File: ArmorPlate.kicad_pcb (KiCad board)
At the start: 2 copper layers, 46 parts, among them SW3 SW_SP3T

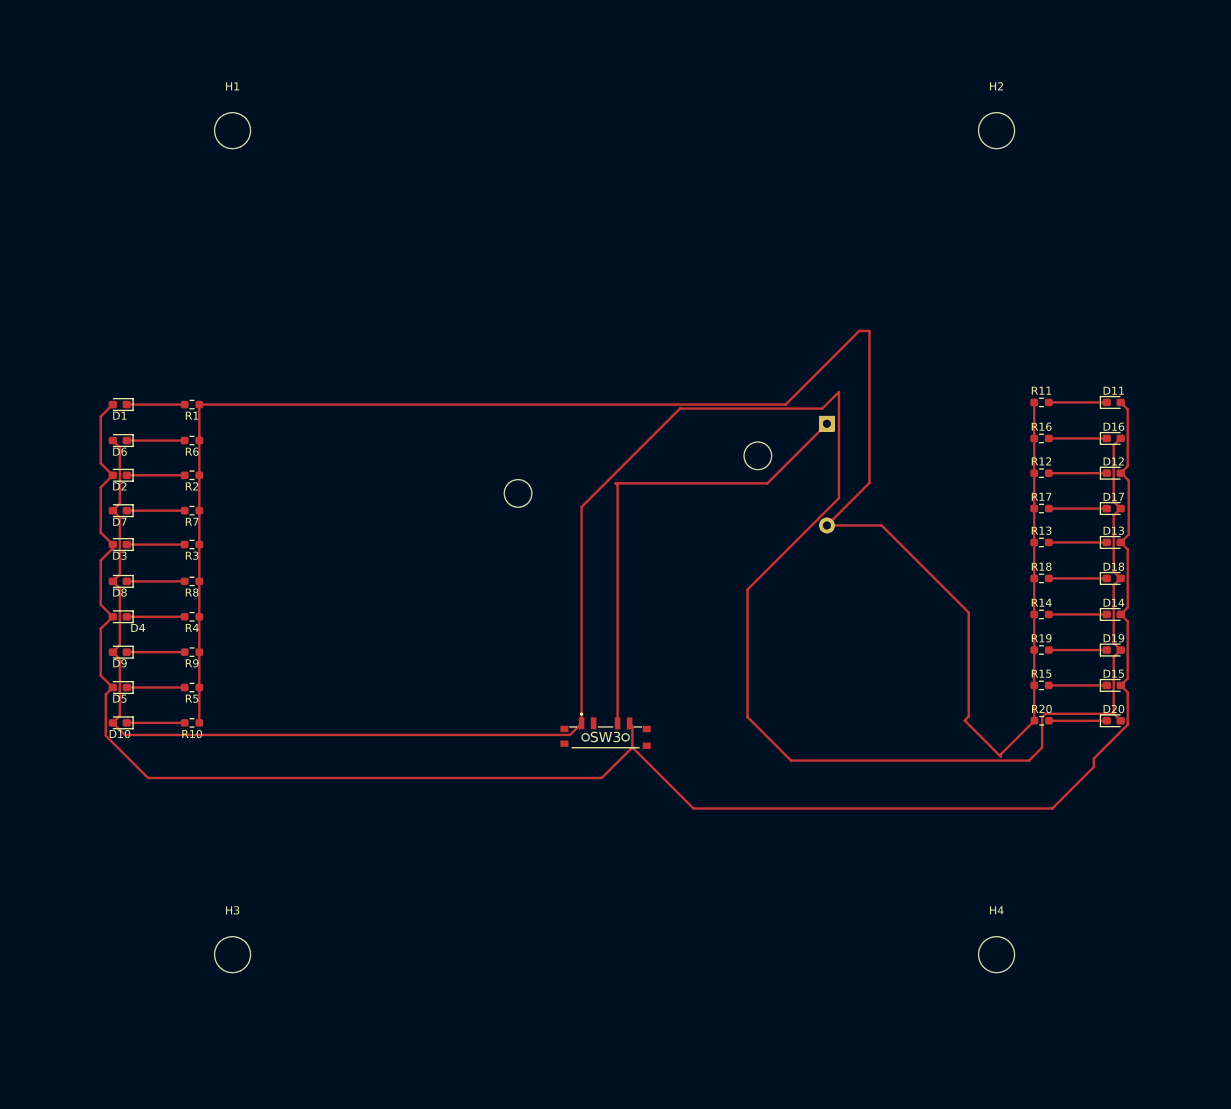
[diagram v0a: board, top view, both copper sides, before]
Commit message: final armorplate pcb with sp3t toggle switch
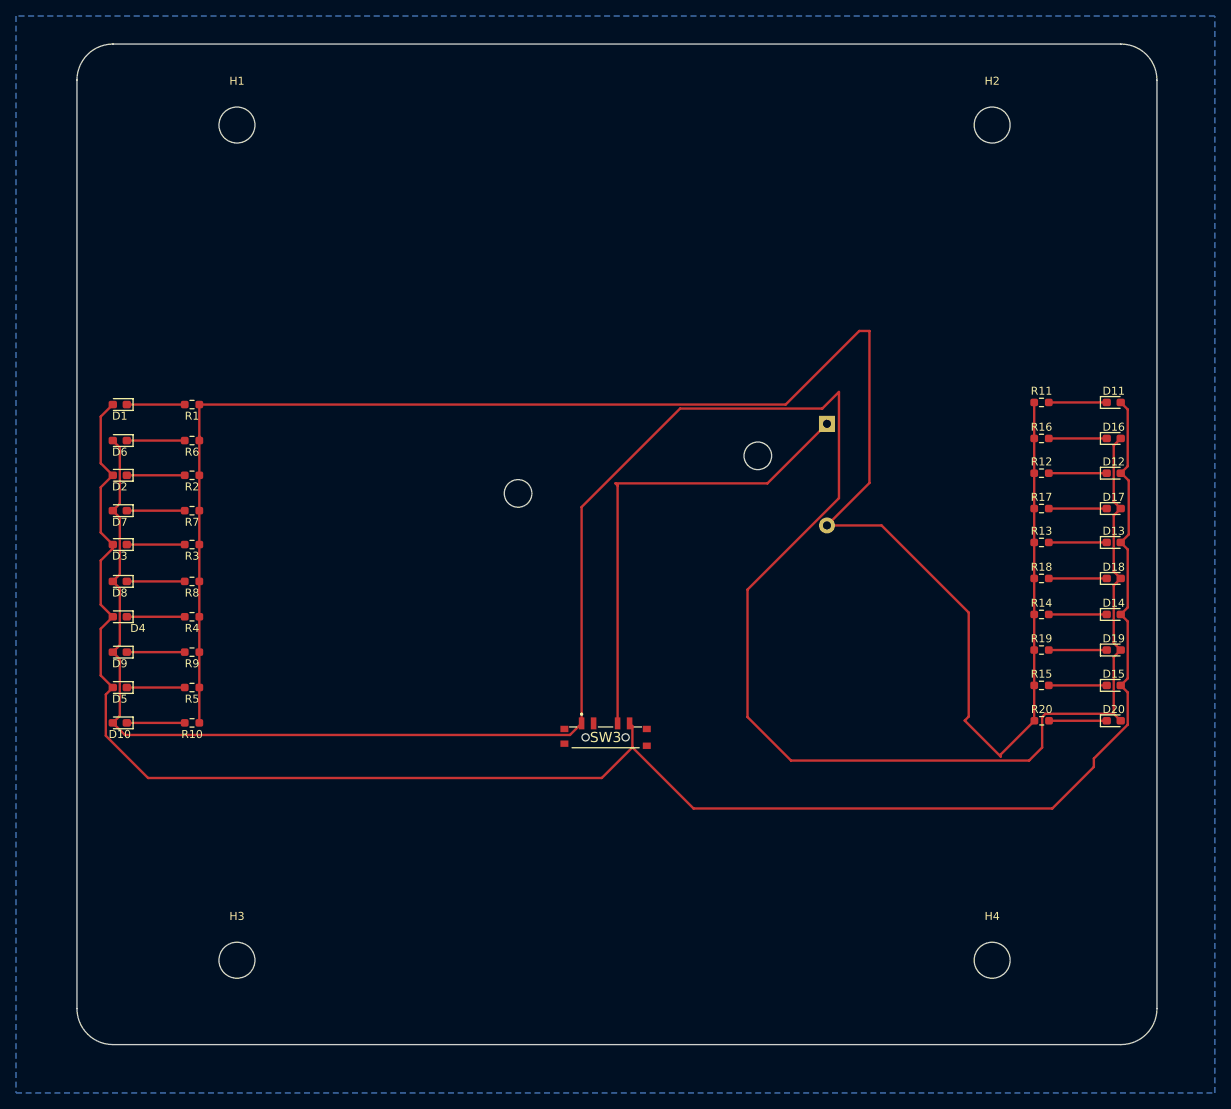
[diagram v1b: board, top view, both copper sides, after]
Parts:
- moved H2 0.89 mm to (196.9, 40.3)
- moved H1 0.89 mm to (102.5, 40.3)
- moved H4 0.89 mm to (196.9, 144.7)
- moved H3 0.89 mm to (102.5, 144.7)
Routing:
- added copper zone on B.Cu, net GND
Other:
- board outline added: 135 x 125.1 mm
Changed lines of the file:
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@@
 	(footprint "MountingHole:MountingHole_4.5mm"
 		(layer "F.Cu")
-		(at 102 144)
+		(at 102.55 144.7)
 		(descr "Mounting Hole 4.5mm, no annular")
 		(tags "mounting hole 4.5mm no annular")
@@
 	(footprint "MountingHole:MountingHole_4.5mm"
 		(layer "F.Cu")
-		(at 102 41)
+		(at 102.55 40.3)
 		(descr "Mounting Hole 4.5mm, no annular")
 		(tags "mounting hole 4.5mm no annular")
@@
 	(footprint "MountingHole:MountingHole_4.5mm"
 		(layer "F.Cu")
-		(at 197.5 41)
+		(at 196.95 40.3)
 		(descr "Mounting Hole 4.5mm, no annular")
 		(tags "mounting hole 4.5mm no annular")
@@
 	(footprint "MountingHole:MountingHole_4.5mm"
 		(layer "F.Cu")
-		(at 197.5 144)
+		(at 196.95 144.7)
 		(descr "Mounting Hole 4.5mm, no annular")
 		(tags "mounting hole 4.5mm no annular")
@@
 		)
 	)
+	(gr_arc
+		(start 217.55 150.745)
+		(mid 216.231981 153.926981)
+		(end 213.05 155.245)
+		(stroke
+			(width 0.05)
+			(type default)
+		)
+		(layer "Edge.Cuts")
+	)
+	(gr_arc
+		(start 213.05 30.175)
+		(mid 216.231981 31.493019)
+		(end 217.55 34.675)
+		(stroke
+			(width 0.05)
+			(type default)
+		)
+		(layer "Edge.Cuts")
+	)
+	(gr_line
+		(start 217.55 34.675)
+		(end 217.55 150.745)
+		(stroke
+			(width 0.05)
+			(type default)
+		)
+		(layer "Edge.Cuts")
+	)
+	(gr_line
+		(start 82.55 150.745)
+		(end 82.55 34.675)
+		(stroke
+			(width 0.05)
+			(type default)
+		)
+		(layer "Edge.Cuts")
+	)
+	(gr_arc
+		(start 82.55 34.675)
+		(mid 83.868019 31.493019)
+		(end 87.05 30.175)
+		(stroke
+			(width 0.05)
+			(type default)
+		)
+		(layer "Edge.Cuts")
+	)
+	(gr_line
+		(start 213.05 155.245)
+		(end 87.05 155.245)
+		(stroke
+			(width 0.05)
+			(type default)
+		)
+		(layer "Edge.Cuts")
+	)
+	(gr_line
+		(start 87.05 30.175)
+		(end 213.05 30.175)
+		(stroke
+			(width 0.05)
+			(type default)
+		)
+		(layer "Edge.Cuts")
+	)
+	(gr_arc
+		(start 87.05 155.245)
+		(mid 83.868019 153.926981)
+		(end 82.55 150.745)
+		(stroke
+			(width 0.05)
+			(type default)
+		)
+		(layer "Edge.Cuts")
+	)
 	(segment
 		(start 97.845 88.503337)
@@
 		(net 24)
 	)
+	(zone
+		(net 1)
+		(net_name "GND")
+		(layer "B.Cu")
+		(hatch edge 0.5)
+		(connect_pads
+			(clearance 0.5)
+		)
+		(min_thickness 0.25)
+		(filled_areas_thickness no)
+		(fill yes
+			(thermal_gap 0.5)
+			(thermal_bridge_width 0.5)
+		)
+		(polygon
+			(pts
+				(xy 74.93 26.67) (xy 74.93 161.29) (xy 224.79 161.29) (xy 224.79 26.67)
+			)
+		)
+	)
 )
